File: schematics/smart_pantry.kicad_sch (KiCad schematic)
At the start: 5 parts, among them J1 Raspberry_Pi_4, U1 HC-SR04, U2 LM2596, U3 SSD1306, U4 WS2812E

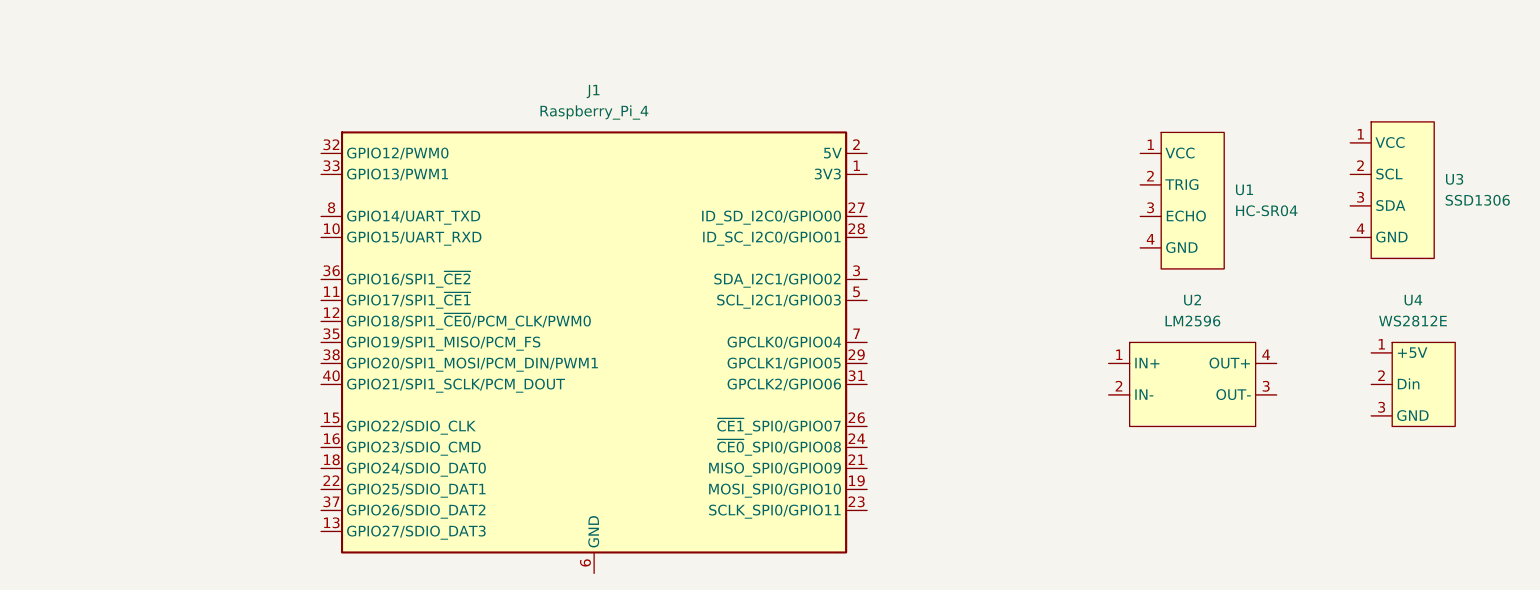
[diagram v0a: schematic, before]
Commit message: Updated KiCAD Schematic
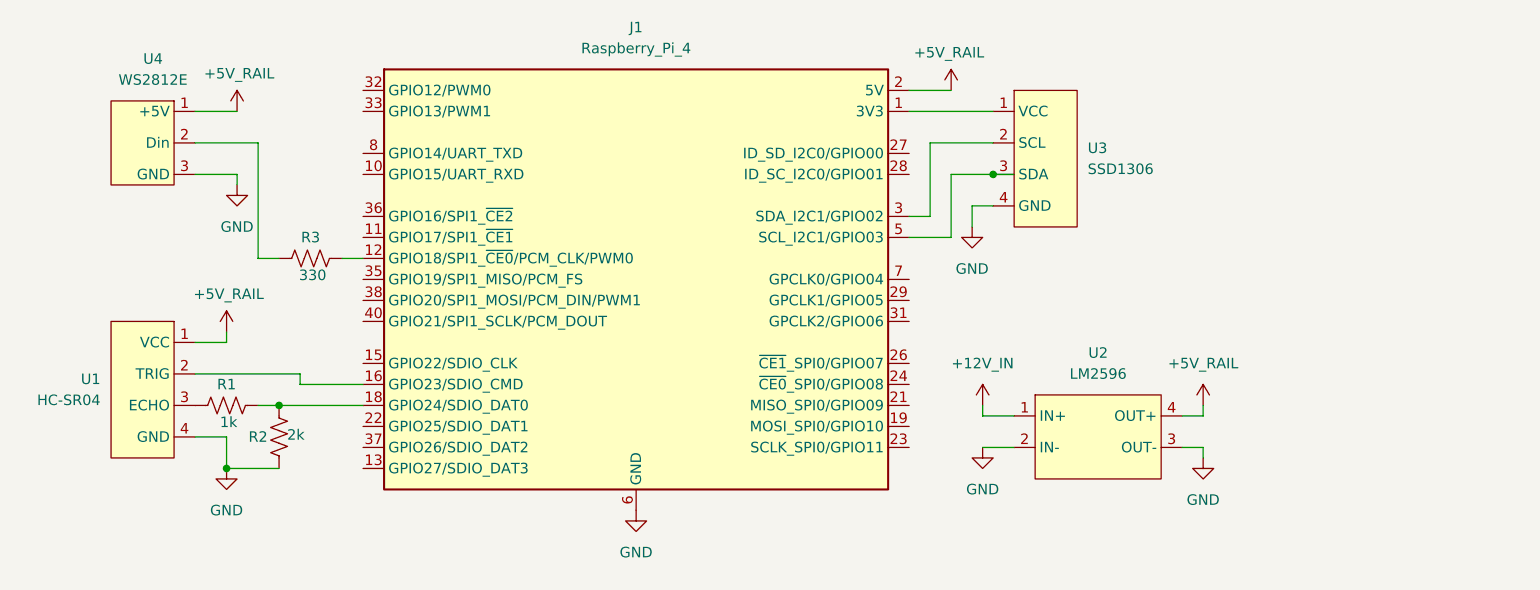
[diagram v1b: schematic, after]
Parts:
- added R1: 1k, symbol Device:R_US
- added R2: 2k, symbol Device:R_US
- added R3: 330, symbol Device:R_US
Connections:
- net +12V_IN: now reaches U2.1 (IN+)
- net GND: now reaches U2.2 (IN-)
- net GND: now also J1.14 (GND), J1.20 (GND), J1.25 (GND), J1.30 (GND), J1.34 (GND), J1.39 (GND), J1.6 (GND), J1.9 (GND), U1.4 (GND), U2.3 (OUT-), U3.4 (GND), U4.3 (GND), R2.1
- net +5V_RAIL: now reaches U2.4 (OUT+)
- net +5V_RAIL: now also J1.2 (5V), J1.4 (5V), U1.1 (VCC), U4.1 (+5V)
- net at U3.1 (VCC): now also J1.1 (3V3), J1.17 (3V3)
- net at U3.2 (SCL): now also J1.3 (SDA_I2C1/GPIO02)
- net at U3.3 (SDA): now also J1.5 (SCL_I2C1/GPIO03)
- net at J1.12 (GPIO18/SPI1_~{CE0}/PCM_CLK/PWM0): now also R3.2
- net at J1.16 (GPIO23/SDIO_CMD): now also U1.2 (TRIG)
- net at J1.18 (GPIO24/SDIO_DAT0): now also R1.2, R2.2
- net at U1.3 (ECHO): now also R1.1
- net at U4.2 (Din): now also R3.1
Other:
- moved on the sheet: J1, U1, U2, U3, U4
